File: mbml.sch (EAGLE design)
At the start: 16 parts, among them IC1 MAX392CPE, J1 CON-2B2B-XH-A(LF)(SN), J2 CON-2B2B-XH-A(LF)(SN), K1 G5SB, Q1 2N2222, X1 43160-1102

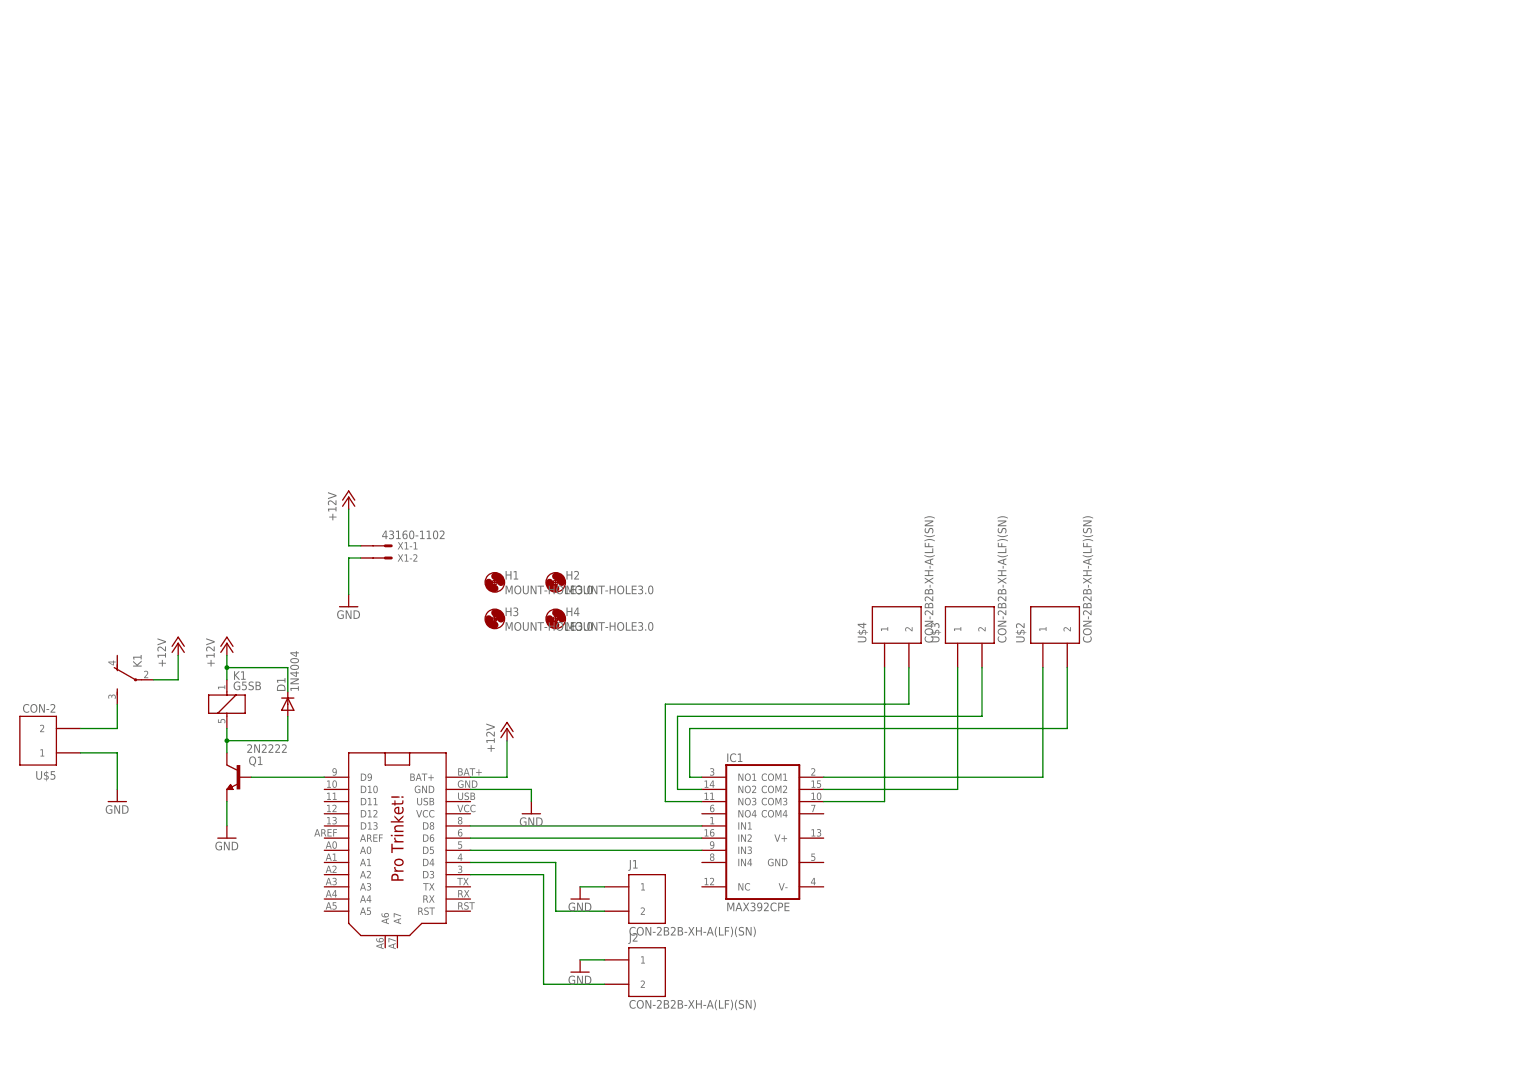
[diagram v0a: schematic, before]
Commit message: Finished board
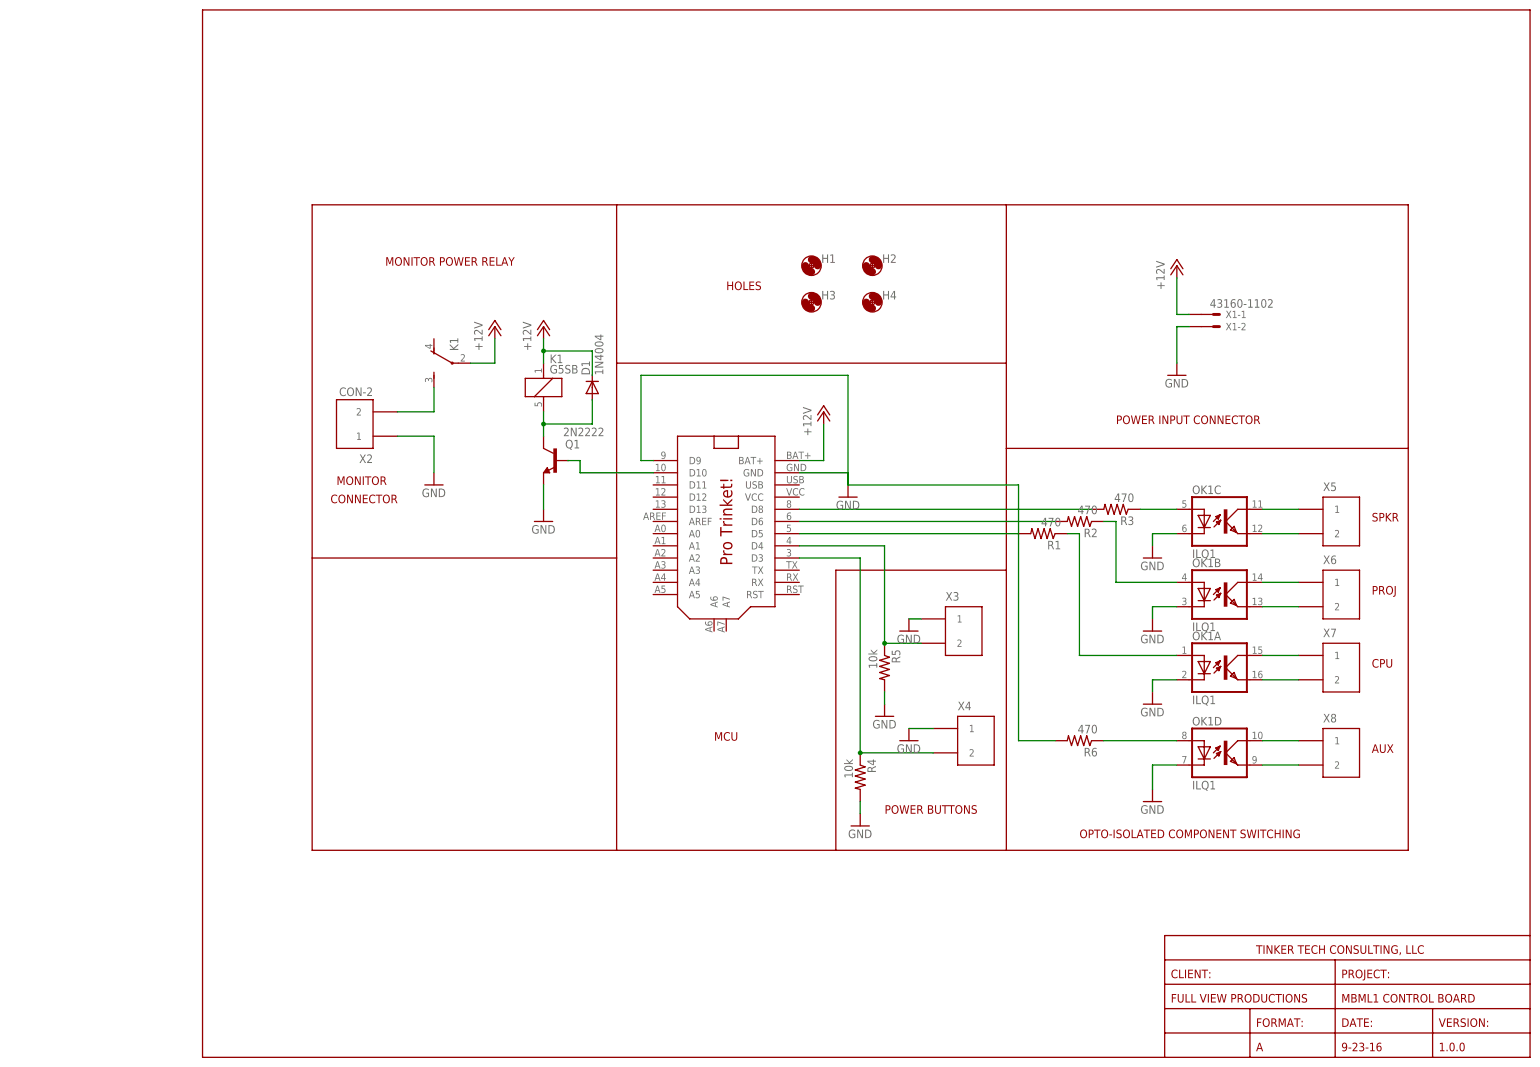
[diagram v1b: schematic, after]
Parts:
- removed IC1: MAX392CPE, maxim:MAX392CPE
- removed J1, J2, U$2, U$3, U$4: CON-2B2B-XH-A(LF)(SN), FVP:CON-2B2B-XH-A(LF)(SN)
- removed U$5: CON-2, FVP:CON-2
- added OK1: ILQ1, optocoupler:ILQ1
- added R1, R2, R3, R6: 470, resistor:R-US_0204/5
- added R4, R5: 10k, resistor:R-US_0204/5
- added X2: CON-2, FVP:CON-2
- added X3, X4, X5, X6, X7, X8: CON-2B2B-XH-A(LF)(SN), FVP:CON-2B2B-XH-A(LF)(SN)
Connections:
- new net N$15: OK1A.COL, X7.1
- new net N$16: OK1A.EMIT, X7.2
- new net N$17: OK1D.A, R6.1
- new net N$18: R6.2, U$1.D9
- new net N$19: OK1D.COL, X8.1
- new net N$20: OK1D.EMIT, X8.2
- new net N$7: OK1B.A, R2.1
- net GND: now also OK1A.C, OK1B.C, OK1C.C, OK1D.C, R4.2, R5.2, X2.1, X3.1, X4.1; no longer J1.1, J2.1, U$5.1
- net MON_PWR: now also X2.2; no longer U$5.2
- net N$1: now also R4.1, X4.2; no longer J2.2
- net N$10: now also R3.2; no longer IC1.IN1
- net N$11: now also OK1C.COL, X5.1; no longer IC1.NO3, U$4.2
- net N$12: now also OK1C.EMIT, X5.2; no longer IC1.COM3, U$4.1
- net N$13: now also OK1B.COL, X6.1; no longer IC1.COM2, U$3.1
- net N$14: now also OK1B.EMIT, X6.2; no longer IC1.COM1, U$2.1
- net N$2: now also R5.1, X3.2; no longer J1.2
- net N$4: now also R1.2; no longer IC1.IN3
- net N$5: now also U$1.D10; no longer U$1.D9
- net N$6: now also OK1C.A, R3.1; no longer IC1.NO1, U$2.2
- net N$8: now also OK1A.A, R1.1; no longer IC1.NO2, U$3.2
- net N$9: now also R2.2; no longer IC1.IN2
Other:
- note added: "1.0.0"
- note added: "9-23-16"
- note added: "A"
- note added: "AUX"
- note added: "CLIENT:"
- note added: "CONNECTOR"
- note added: "CPU"
- note added: "DATE:"
- note added: "FORMAT:"
- note added: "FULL VIEW PRODUCTIONS"
- note added: "HOLES"
- note added: "MBML1 CONTROL BOARD"
- note added: "MCU"
- note added: "MONITOR"
- note added: "MONITOR POWER RELAY"
- note added: "OPTO-ISOLATED COMPONENT SWITCHING"
- note added: "POWER BUTTONS"
- note added: "POWER INPUT CONNECTOR"
- note added: "PROJ"
- note added: "PROJECT:"
- note added: "SPKR"
- note added: "TINKER TECH CONSULTING, LLC"
- note added: "VERSION:"
- moved on the sheet: D1, H1, H2, H3, H4, K1, Q1, X1-1, X1-2
